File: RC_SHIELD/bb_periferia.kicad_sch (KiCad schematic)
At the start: 58 parts, among them J10 POWER_SUPPLY, J11 ALF_MOT_DRV, J11 GPIO1, J12 BET_MOT_DRV, J12 GPIO2, J13 SPI, J14 I2C_TEMP, J15 DOOR_SWITCH, J16 ESTOP, J17 FAN, J18 P5a, J9 P4a, Q1 BSS123, Q2 BSS123, U2 SN75LBC179AD, U3 ESP8266-01/ESP-01, U4 LCD-016N002L

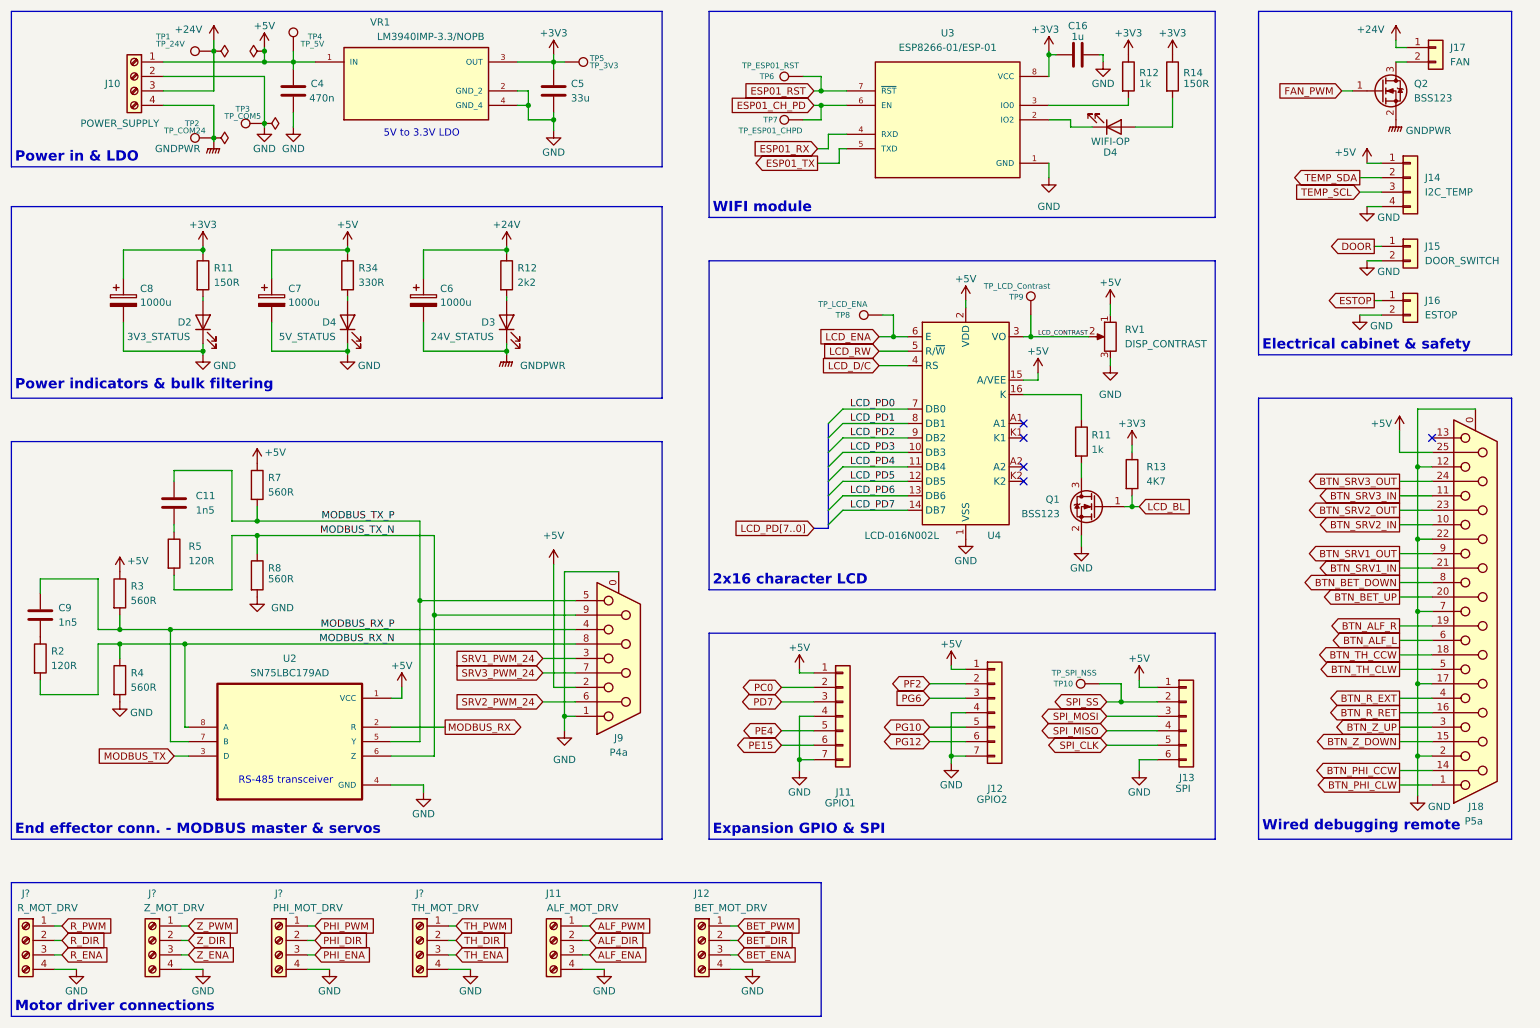
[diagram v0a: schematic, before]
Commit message: [SCH] reannotated entire schematic so PCBnew wont complain
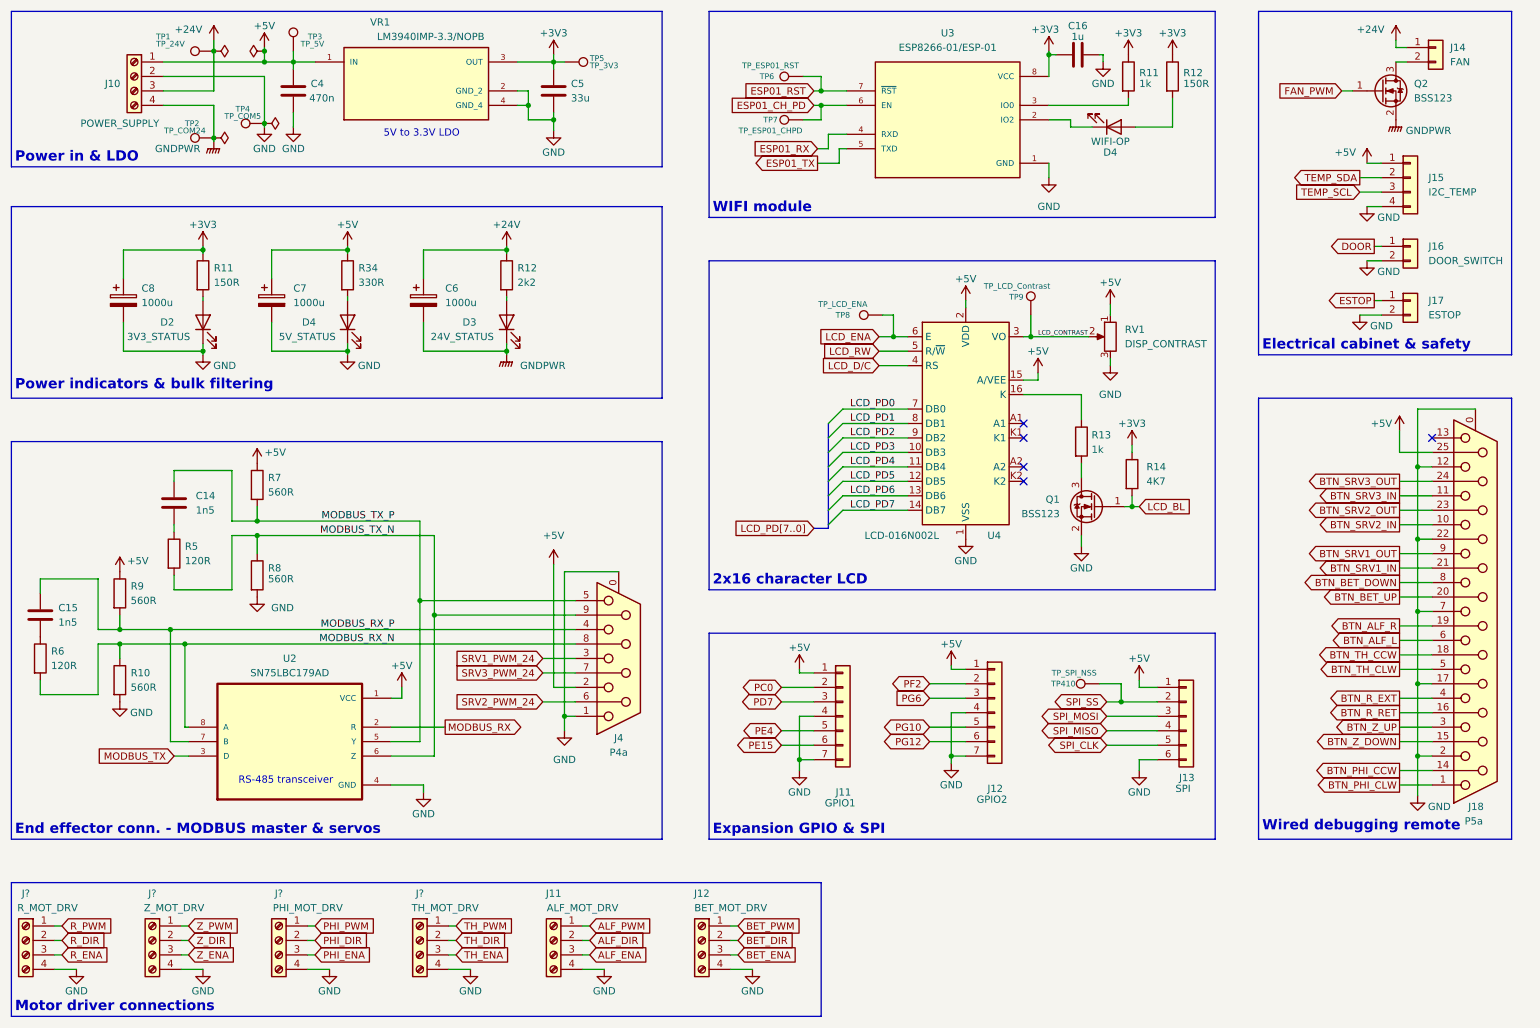
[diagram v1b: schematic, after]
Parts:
- renumbered C11 to C14, C9 to C15, J17 to J14, J14 to J15, J15 to J16, J16 to J17, J9 to J4, R4 to R10, R12 to R11, R14 to R12, R11 to R13, R13 to R14, R2 to R6, R3 to R9, TP4 to TP3, TP3 to TP4, TP10 to TP410

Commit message: Revert "[SCH] reannotated entire schematic so PCBnew wont complain"
This reverts commit df148950bb8496d2d5af5a937770664cb0004a0d.
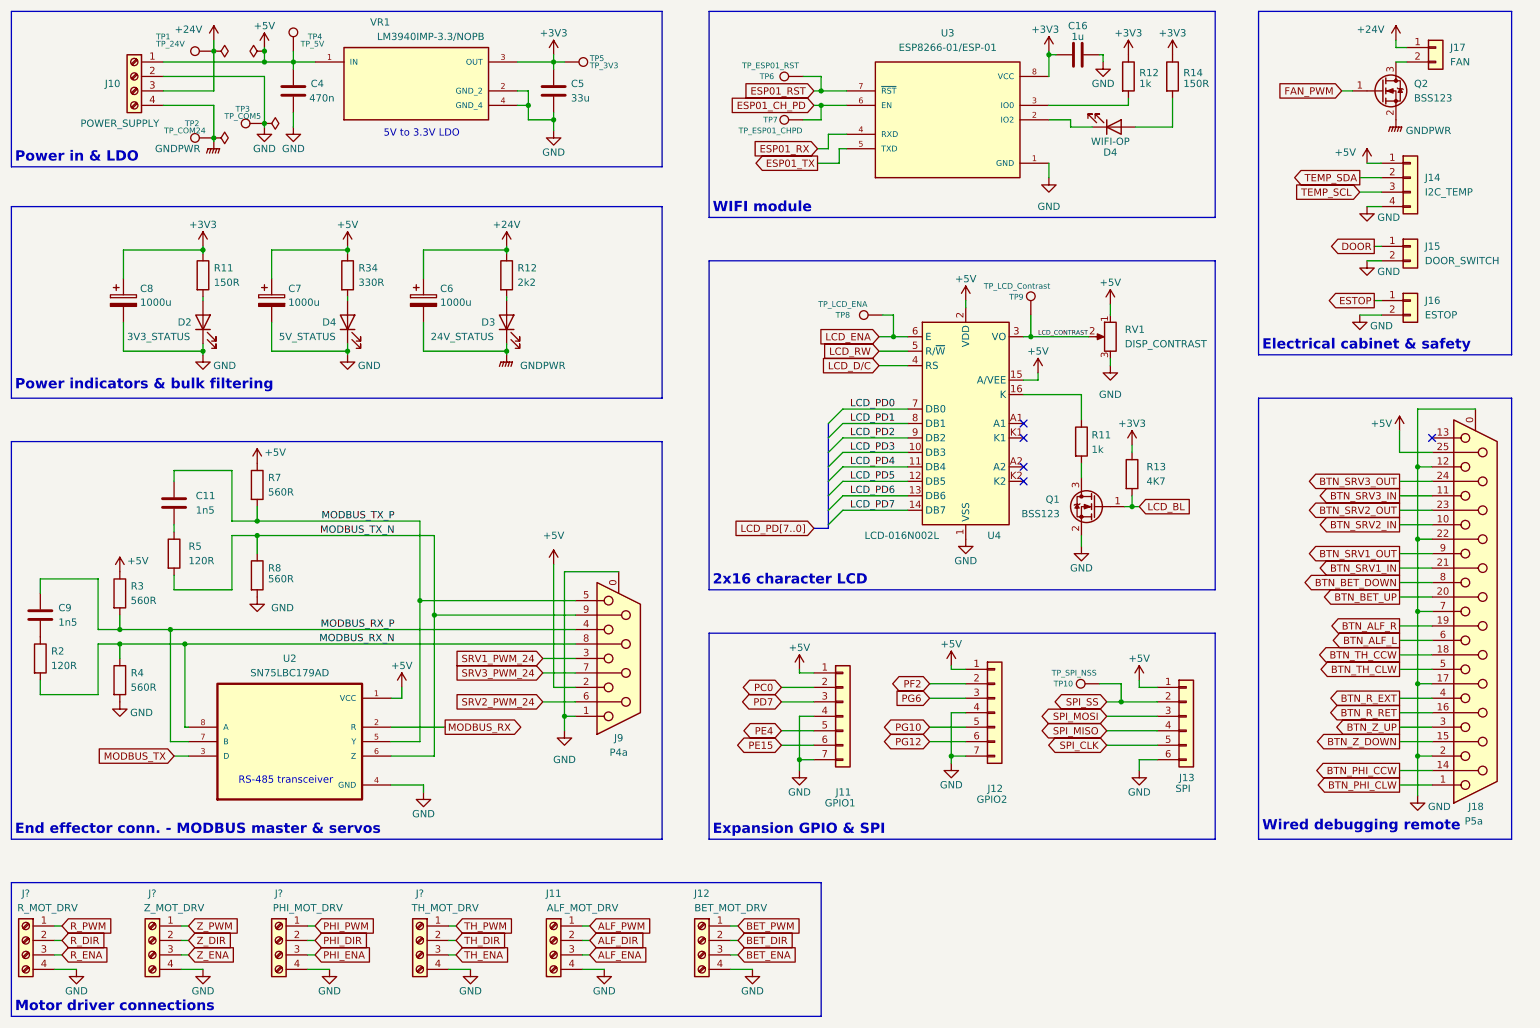
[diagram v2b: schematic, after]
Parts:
- renumbered C14 to C11, C15 to C9, J15 to J14, J16 to J15, J17 to J16, J14 to J17, J4 to J9, R13 to R11, R11 to R12, R14 to R13, R12 to R14, R6 to R2, R9 to R3, R10 to R4, TP410 to TP10, TP4 to TP3, TP3 to TP4
